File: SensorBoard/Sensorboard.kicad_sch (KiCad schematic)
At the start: 56 parts, among them J1 Conn_01x16_Pin, U1 LM339, U10 LM339, U2 CNY70, U3 CNY70, U4 CNY70, U5 CNY70, U6 CNY70, U7 CNY70, U8 CNY70

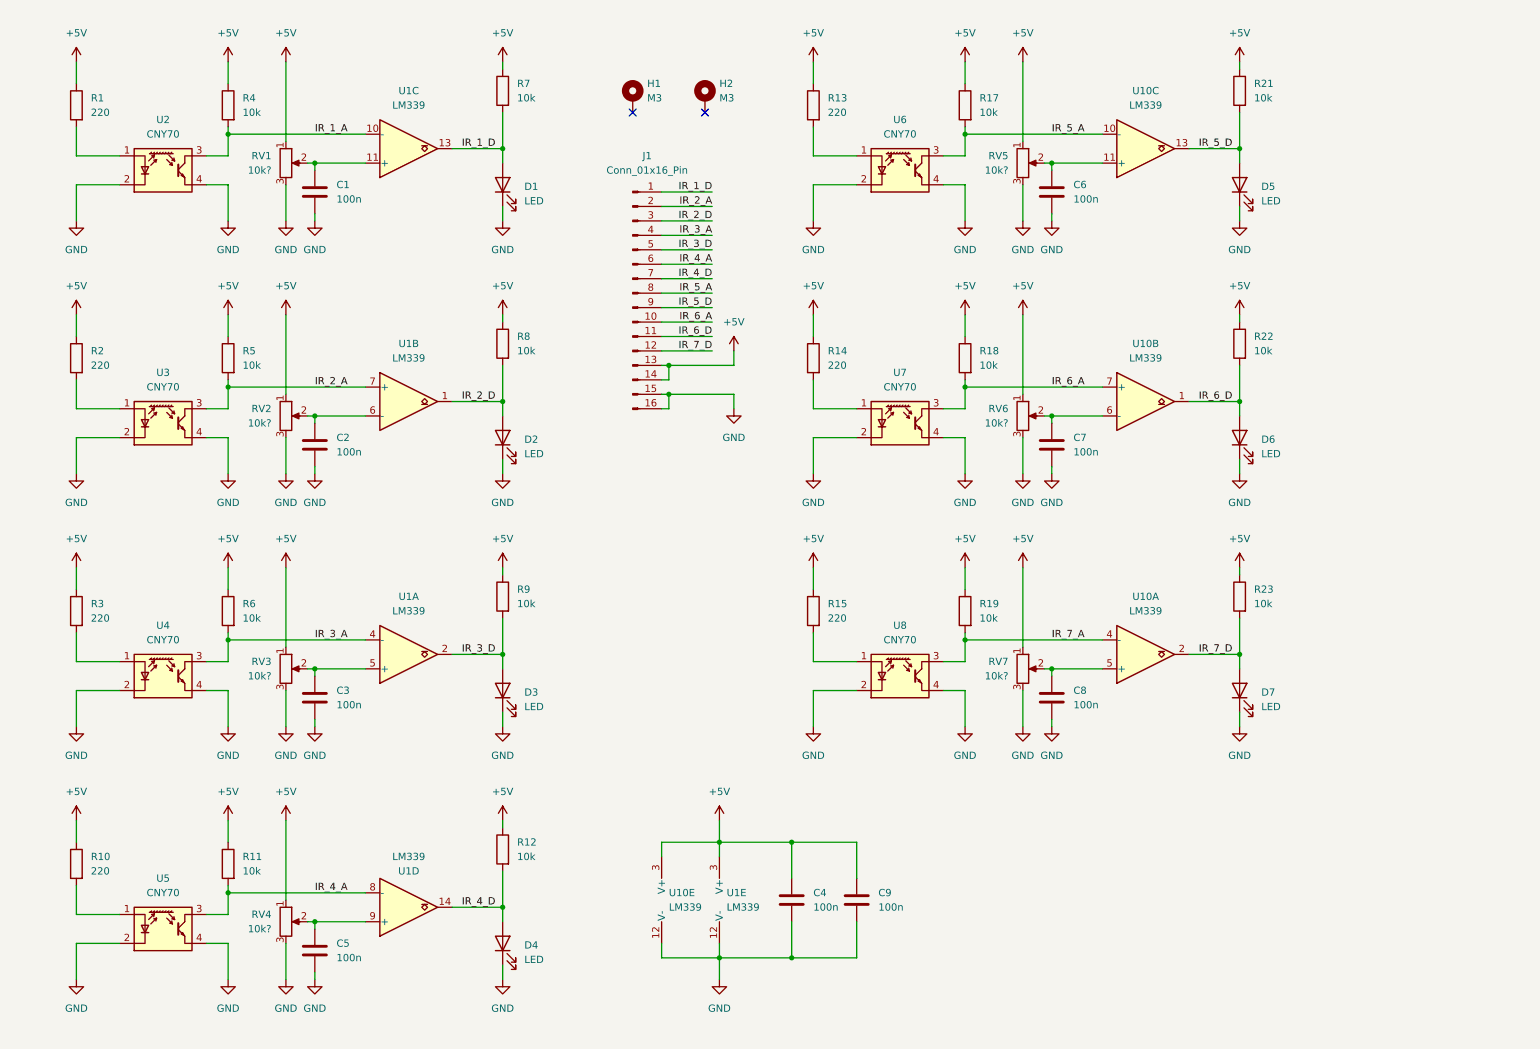
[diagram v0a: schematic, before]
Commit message: SensorBoard Updates
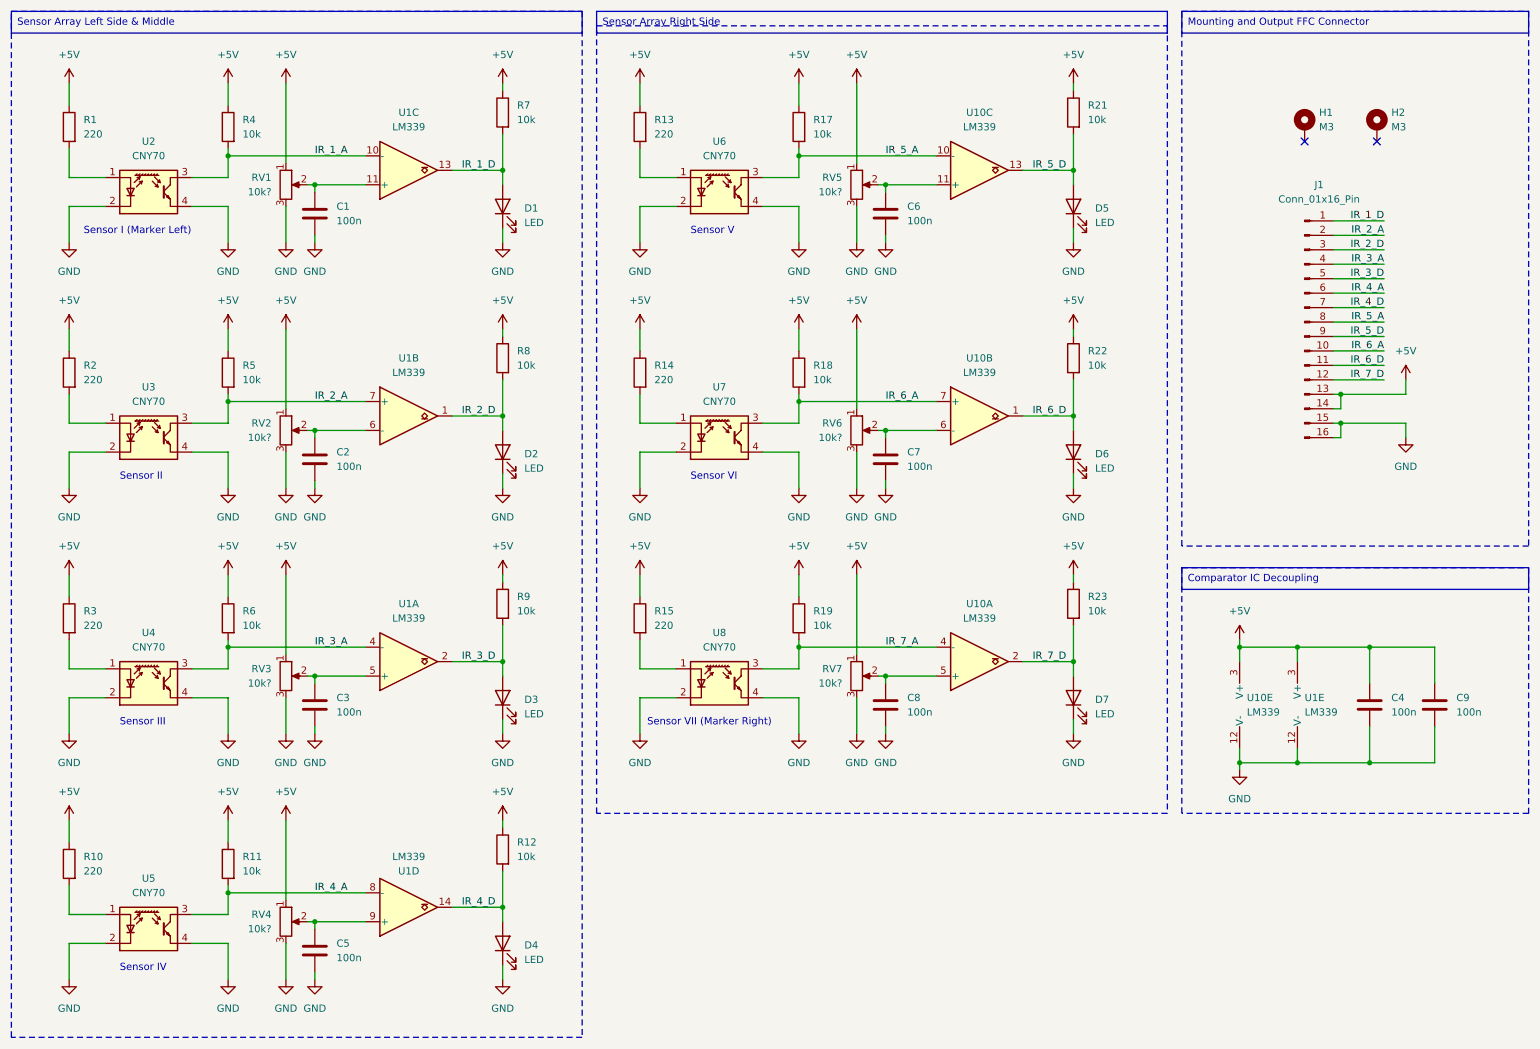
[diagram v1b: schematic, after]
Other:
- note added: "Sensor I (Marker Left)"
- note added: "Sensor II"
- note added: "Sensor III"
- note added: "Sensor IV"
- note added: "Sensor V"
- note added: "Sensor VI"
- note added: "Sensor VII (Marker Right)"
- moved on the sheet: C1, C2, C3, C4, C6, C7, C8, C9, D1, D2, D3, D5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
